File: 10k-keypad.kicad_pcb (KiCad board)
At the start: 2 copper layers, 42 parts, among them J1 AVR-ISP-6, K1 SW_Push, K10 SW_Push, K2 SW_Push, K3 SW_Push, K4 SW_Push, K5 SW_Push, K6 SW_Push, K7 SW_Push, K8 SW_Push, K9 SW_Push, SW1 SW_Push, U1 ATmega16U2-A, Y1 Crystal_GND24_Small

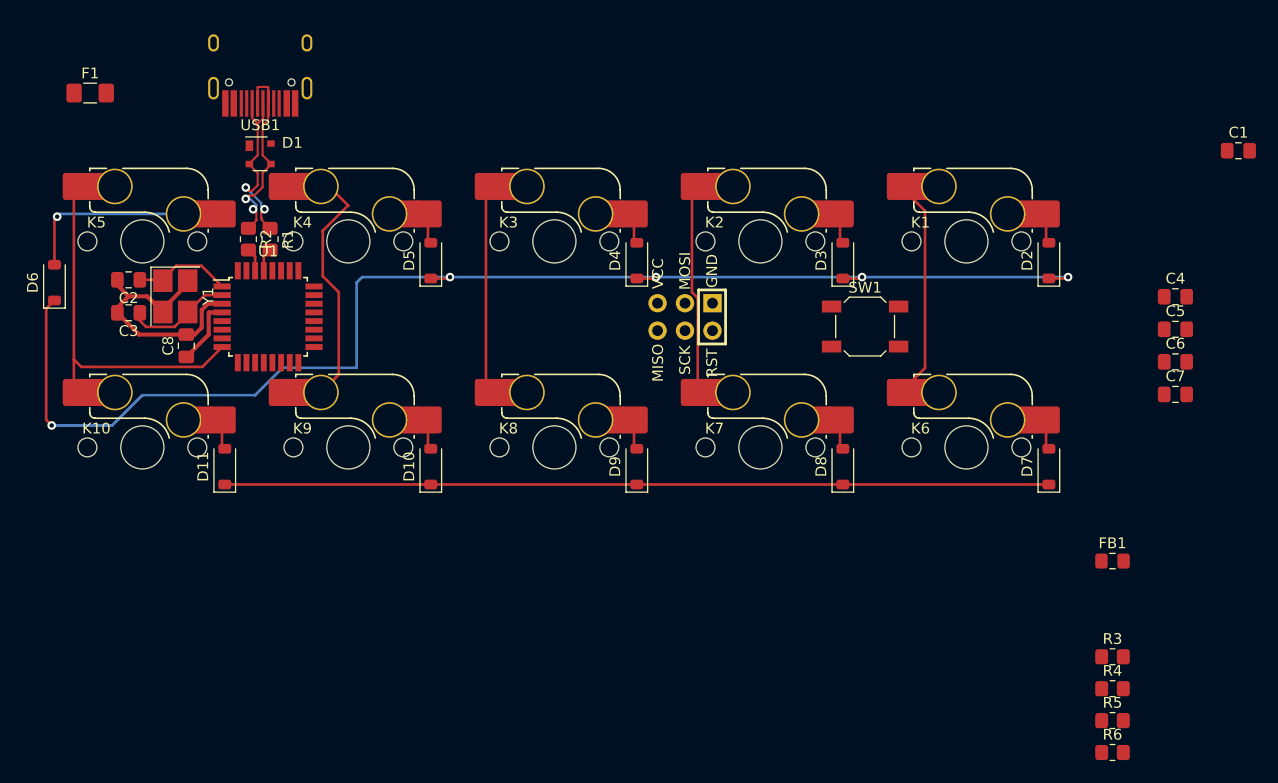
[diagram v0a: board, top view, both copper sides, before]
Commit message: finish routing
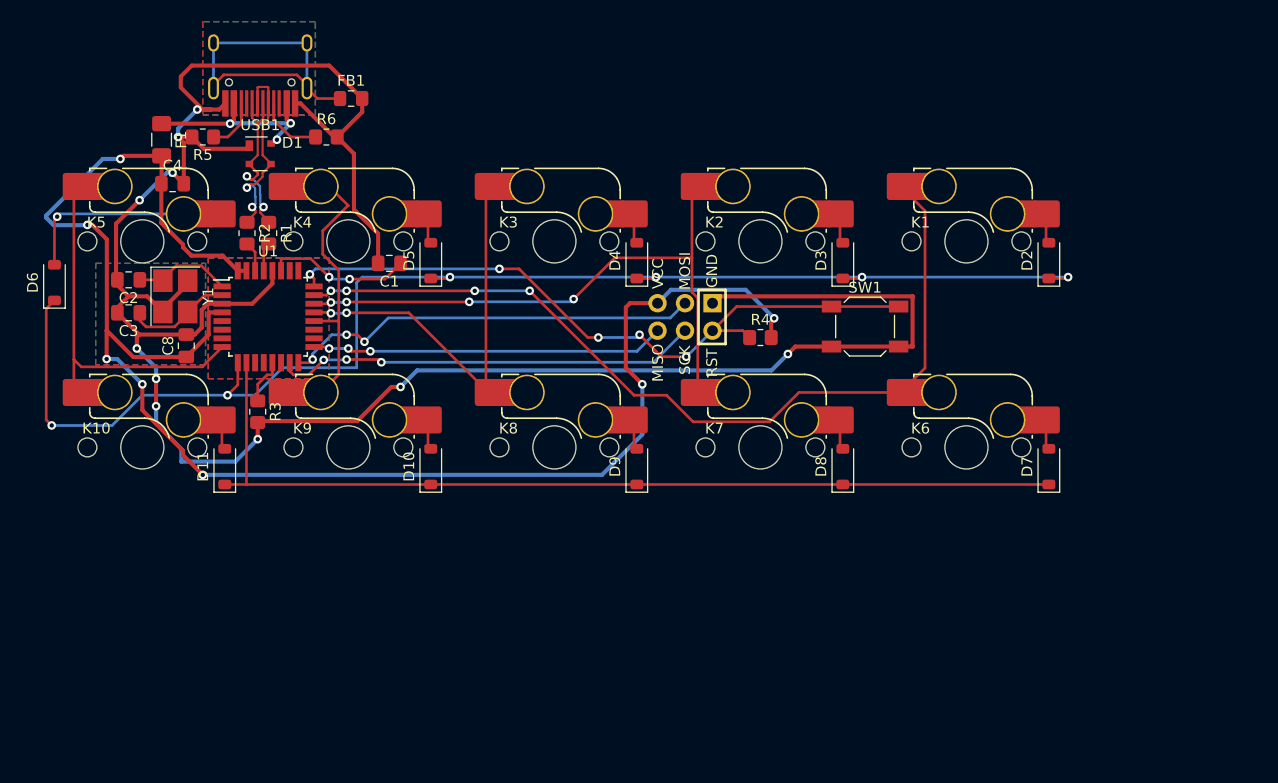
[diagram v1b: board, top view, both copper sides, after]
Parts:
- removed C5, C6, C7: 0.1u, Capacitor_SMD:C_0805_2012Metric_Pad1.18x1.45mm_HandSolder
- moved R5 99.9 mm to (148.8, 26.4), turned to 180 degrees
- moved C4 93.3 mm to (146.1, 30.7)
- moved R6 92.3 mm to (160.3, 26.4)
- moved FB1 82.4 mm to (162.6, 22.9)
- moved R3 82.2 mm to (153.9, 51.8), turned to -90 degrees
- moved C1 79.2 mm to (166.1, 38.1), turned to 180 degrees
- moved R4 46.0 mm to (200.4, 45.0)
- moved F1 7.89 mm to (145.0, 26.7), turned to -90 degrees
- moved R1 0.57 mm to (154.9, 35.3)
- moved R2 0.57 mm to (152.9, 35.3)
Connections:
- U1 pad 10: unconnected-(U1-PD4-Pad10) -> ROW2
- U1 pad 20: unconnected-(U1-PB6-Pad20) -> COL4
- U1 pad 21: unconnected-(U1-PB7-Pad21) -> COL3
- U1 pad 22: COL4 -> COL2
- U1 pad 23: COL3 -> COL1
- U1 pad 25: COL2 -> unconnected-(U1-PC5-Pad25)
- U1 pad 26: COL1 -> unconnected-(U1-PC4-Pad26)
- U1 pad 6: ROW2 -> unconnected-(U1-PD0-Pad6)
- U1 pad 7: ROW1 -> unconnected-(U1-PD1-Pad7)
- U1 pad 9: unconnected-(U1-PD3-Pad9) -> ROW1
- USB1 pad 13: GND -> Earth
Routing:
- net GND: track 24.2 -> 218.4 mm, vias 0 -> 10
- net +5V: track 6.22 -> 148.3 mm, vias 0 -> 7
- net RESET: track 0.00 -> 65.1 mm, vias 0 -> 5
- net COL1: track 20.9 -> 81.5 mm, vias 0 -> 4
- net SCK: track 0.00 -> 39.4 mm, vias 0 -> 3
- net MOSI: track 0.00 -> 38.9 mm, vias 0 -> 3
- net COL2: track 19.5 -> 56.2 mm, vias 0 -> 4
- net MISO: track 0.00 -> 32.7 mm, vias 0 -> 3
- net Earth: track 0.00 -> 30.5 mm
- net COL3: track 19.2 -> 38.5 mm, vias 0 -> 2
- net VCC: track 0.00 -> 18.7 mm, vias 0 -> 3
- net Net-(U1-UCAP): track 0.00 -> 13.5 mm, vias 0 -> 2
- net ROW2: track 76.2 -> 87.5 mm
- net Net-(USB1-CC1): track 0.00 -> 6.05 mm
- net Net-(USB1-CC2): track 0.00 -> 4.94 mm
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- added copper zone on B.Cu, net Earth
- added copper zone on F.Cu, net Earth
- added copper zone on B.Cu, net GND
- added copper zone on F.Cu, net GND
